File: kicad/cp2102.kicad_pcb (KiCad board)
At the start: 2 copper layers, 21.3 x 14.2 mm, 10 parts, among them P1 CONN_01X05, P2 MICRO-USB-B, U1 CP2102

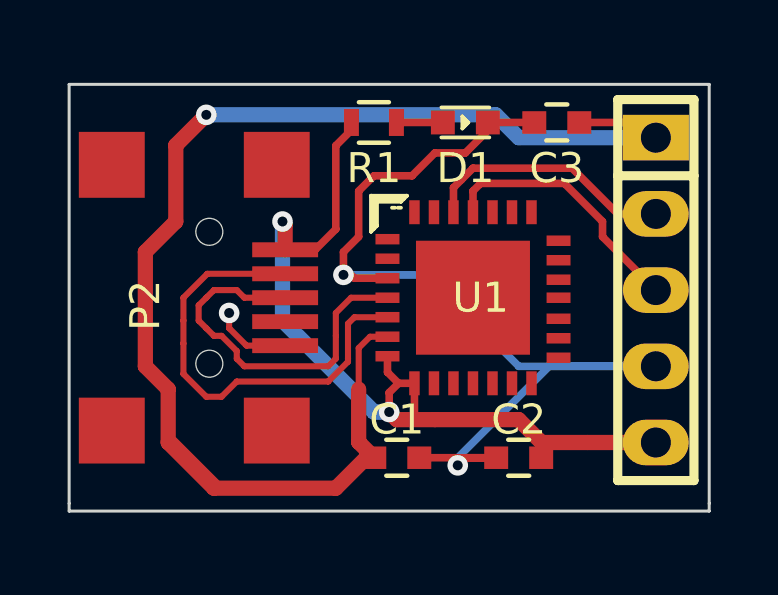
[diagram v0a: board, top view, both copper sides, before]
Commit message: ver2.0
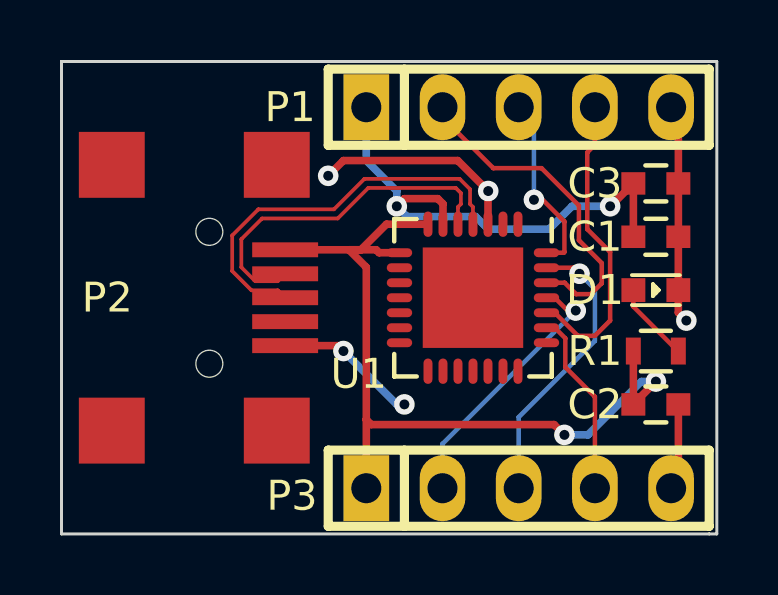
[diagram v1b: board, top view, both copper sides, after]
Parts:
- removed LOGO2: OPEN_HARDWARE_1, BASIC:LOGO_SILK_OSHW_6x6mm
- added P3: CONN_01X05, BASIC:PIN_SOCKET_5, F.Cu at (203.2, 157.2)
- U1: footprint BASIC:QFN-28 -> BASIC:QFN-28-1EP_5x5mm_Pitch0.5mm
- moved R1 12.1 mm to (207.8, 152.7)
- moved C1 11.4 mm to (207.8, 148.8)
- moved LOGO1 8.89 mm to (195.3, 153.4), turned to 90 degrees
- moved D1 8.46 mm to (207.8, 150.6)
- moved P1 7.62 mm to (203.2, 144.5), turned to 0 degrees
- moved C2 4.91 mm to (207.8, 154.4), turned to 0 degrees
- moved C3 3.88 mm to (207.8, 147.1), turned to 0 degrees
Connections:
- P1 pad 3: /RXD -> /DTR
- P1 pad 4: GND -> /RTS
- P1 pad 5: VCC -> GND
- P2 pad 4: (no net) -> Net-(P2-Pad4)
- U1 pad 1: (no net) -> Net-(U1-Pad1)
- U1 pad 11: (no net) -> Net-(U1-Pad11)
- U1 pad 12: (no net) -> Net-(U1-Pad12)
- U1 pad 2: (no net) -> Net-(U1-Pad2)
- U1 pad 23: (no net) -> /CTS
- U1 pad 24: (no net) -> /RTS
- U1 pad 27: (no net) -> /DSR
- U1 pad 28: (no net) -> /DTR
- U1 pad 9: (no net) -> Net-(U1-Pad9)
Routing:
- net +3V3: track 65.7 -> 17.4 mm, vias 1 -> 2
- net GND: track 37.9 -> 22.1 mm, vias 3 -> 5
- net /RTS: track 0.00 -> 10.2 mm
- net /DSR: track 0.00 -> 9.60 mm, vias 0 -> 1
- net /DTR: track 0.00 -> 6.27 mm, vias 0 -> 1
- net /CTS: track 0.00 -> 6.18 mm
- net VCC: track 31.9 -> 28.5 mm
- net /D-: track 15.2 -> 11.9 mm
- net /TXD: track 9.73 -> 11.2 mm
- net Net-(D1-Pad1): track 1.55 -> 2.66 mm
- net /D+: track 12.6 -> 13.4 mm
- net /RXD: track 8.68 -> 8.98 mm, vias 0 -> 1
- added copper zone on F.Cu, net GND
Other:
- board size 21.3 x 14.2 mm -> 21.8 x 15.7 mm
- net class Default: trace_width 0.204 -> 0.1524
- rule trace_min: 0.127 -> 0.125
- board text added: "3V3"
- board text added: "5V"
- board text added: "CTS"
- board text added: "DSR"
- board text added: "DTR"
- board text added: "GND"
- board text added: "RTS"
- board text added: "RXD"
- board text added: "TXD"
